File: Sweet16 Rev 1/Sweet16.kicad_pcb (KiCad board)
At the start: 2 copper layers, 140 x 60 mm, 113 parts, among them J1 Conn_01x09_Male, J10 SW_half_inverter, J11 R_clock, J12 OUT_clock, J13 SW_dual8_hex, J14 OUT_OUT, J15 R_sync_pitch_1, J16 SW_sync_1, J17 R_sync_pitch_2, J18 SW_sync_2, J2 Conn_01x09_Male, J20 R_sync_pitch_2, J21 SW_dual8_hex_2, J22 OUT_OUT, J23 OUT_CARRY_OUT, J3 Conn_01x09_Male, J4 Conn_01x09_Male, J5 OUT_OUT, J6 SW_run, J7 SW_BIN_DEC, J8 SW_UP_DN, J9 SW_clock_source, U1 40106, U2 4029, U3 4028, U4 4051, U5 4028, U6 4070, U7 4051, U8 LM358

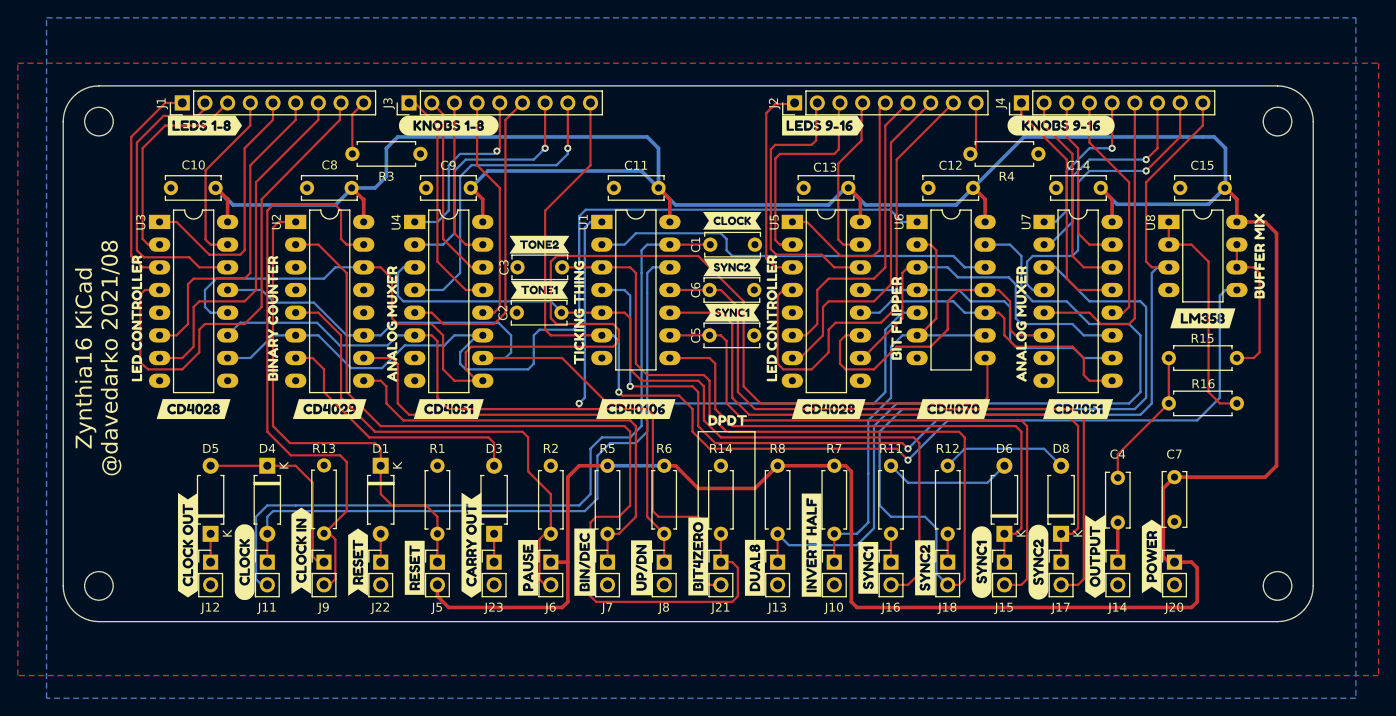
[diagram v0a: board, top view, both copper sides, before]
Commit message: moved the pulldown where it would work
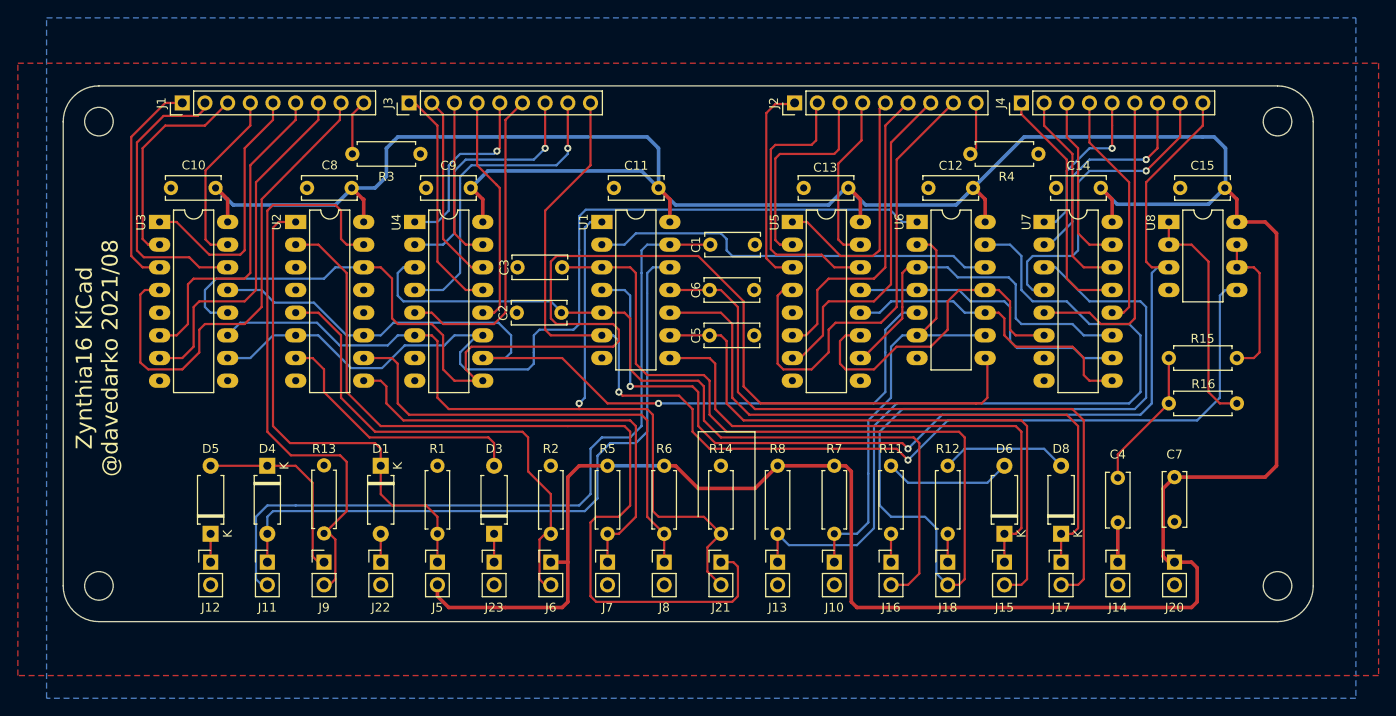
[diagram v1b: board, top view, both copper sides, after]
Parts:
- removed kibuzzard-610C1637, kibuzzard-610C1856, kibuzzard-610C1A63, kibuzzard-610C1AC8, kibuzzard-610C1D73, kibuzzard-610C1E26, kibuzzard-610C2350, kibuzzard-610C23E8, kibuzzard-610C2455, kibuzzard-610C51A7, kibuzzard-610C51E0, kibuzzard-610C523D, kibuzzard-610C5269, kibuzzard-610C52EC, kibuzzard-610C530B, kibuzzard-610C5339, kibuzzard-610C5373, kibuzzard-610C5418, kibuzzard-610C545E, kibuzzard-610C5562, kibuzzard-610C55EA, kibuzzard-610C561B, kibuzzard-6111A8BD, kibuzzard-6112EA2B, kibuzzard-6112EA3D, kibuzzard-6112EA56, kibuzzard-6112EA78, kibuzzard-6112EA8E, kibuzzard-6112EAB9, kibuzzard-6112EAC9, kibuzzard-6112EADF, kibuzzard-6112EDB2, kibuzzard-6112EDD8, kibuzzard-6112EDF7, kibuzzard-6112EE23, kibuzzard-6112EE9D, kibuzzard-6112EEB7, kibuzzard-6112EED9, kibuzzard-6112EEFB, kibuzzard-6112F4A3, kibuzzard-6112F4D1, kibuzzard-6112F4F2, kibuzzard-6112F51D, kibuzzard-6112F530: G***, label
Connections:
- R14 pad 1: QD0 -> QD1
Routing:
- net QD0: track 101.3 -> 98.2 mm
- net QD1: track 105.4 -> 106.3 mm

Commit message: Revert "moved the pulldown where it would work"
This reverts commit ad45cd7af2cd5e29d93eb6355ad2eb9f66b6a434.
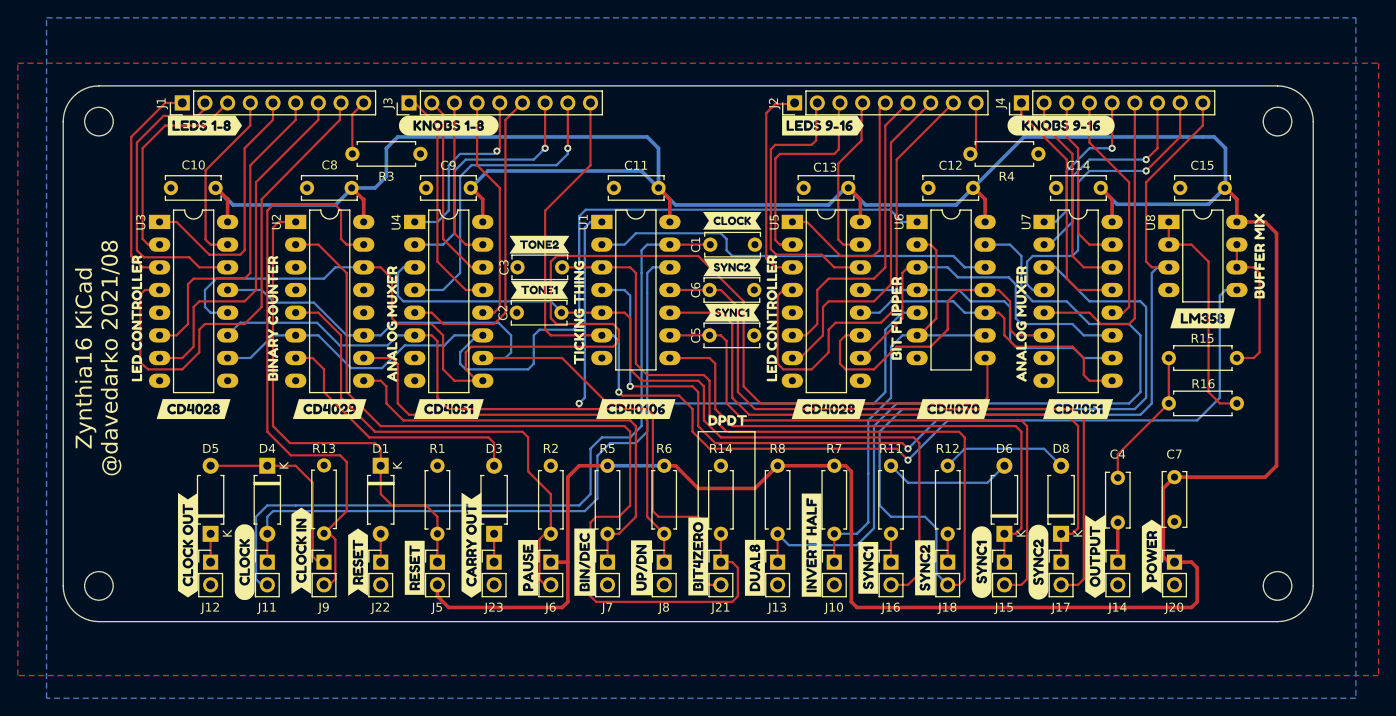
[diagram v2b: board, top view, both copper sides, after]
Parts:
- added kibuzzard-610C1637: G***, label, F.Cu at (45.7, 51.4)
- added kibuzzard-610C1856: G***, label, F.Cu at (64.8, 54.0)
- added kibuzzard-610C1A63: G***, label, F.Cu at (58.4, 53.3)
- added kibuzzard-610C1AC8: G***, label, F.Cu at (83.8, 51.4)
- added kibuzzard-610C1D73: G***, label, F.Cu at (39.4, 54.0)
- added kibuzzard-610C1E26: G***, label, F.Cu at (33.0, 53.3)
- added kibuzzard-610C2350: G***, label, F.Cu at (77.5, 54.0)
- added kibuzzard-610C23E8: G***, label, F.Cu at (71.1, 52.7)
- added kibuzzard-610C2455: G***, label, F.Cu at (74.4, 37.5)
- added kibuzzard-610C51A7: G***, label, F.Cu at (90.2, 54.0)
- added kibuzzard-610C51E0: G***, label, F.Cu at (96.5, 54.0)
- added kibuzzard-610C523D: G***, label, F.Cu at (109.2, 53.3)
- added kibuzzard-610C5269: G***, label, F.Cu at (102.9, 53.3)
- added kibuzzard-610C52EC: G***, label, F.Cu at (15.9, 4.45)
- added kibuzzard-610C530B: G***, label, F.Cu at (85.1, 4.45)
- added kibuzzard-610C5339: G***, label, F.Cu at (111.8, 4.45)
- added kibuzzard-610C5373: G***, label, F.Cu at (43.2, 4.45)
- added kibuzzard-610C5418: G***, label, F.Cu at (14.0, 51.4)
- added kibuzzard-610C545E: G***, label, F.Cu at (26.7, 52.1)
- added kibuzzard-610C5562: G***, label, F.Cu at (20.3, 53.3)
- added kibuzzard-610C55EA: G***, label, F.Cu at (52.1, 54.0)
- added kibuzzard-610C561B: G***, label, F.Cu at (115.6, 52.7)
- added kibuzzard-6111A8BD: G***, label, F.Cu at (121.9, 52.7)
- added kibuzzard-6112EA2B: G***, label, F.Cu at (14.6, 36.2)
- added kibuzzard-6112EA3D: G***, label, F.Cu at (85.7, 36.2)
- added kibuzzard-6112EA56: G***, label, F.Cu at (29.8, 36.2)
- added kibuzzard-6112EA78: G***, label, F.Cu at (43.2, 36.2)
- added kibuzzard-6112EA8E: G***, label, F.Cu at (113.7, 36.2)
- added kibuzzard-6112EAB9: G***, label, F.Cu at (64.1, 36.2)
- added kibuzzard-6112EAC9: G***, label, F.Cu at (99.7, 36.2)
- added kibuzzard-6112EADF: G***, label, F.Cu at (127.6, 26.0)
- added kibuzzard-6112EDB2: G***, label, F.Cu at (8.26, 26.0)
- added kibuzzard-6112EDD8: G***, label, F.Cu at (23.5, 26.0)
- added kibuzzard-6112EDF7: G***, label, F.Cu at (36.8, 26.7)
- added kibuzzard-6112EE23: G***, label, F.Cu at (107.3, 26.7)
- added kibuzzard-6112EE9D: G***, label, F.Cu at (57.8, 25.4)
- added kibuzzard-6112EEB7: G***, label, F.Cu at (79.4, 26.0)
- added kibuzzard-6112EED9: G***, label, F.Cu at (134.0, 19.1)
- added kibuzzard-6112EEFB: G***, label, F.Cu at (93.3, 26.0)
- added kibuzzard-6112F4A3: G***, label, F.Cu at (74.9, 15.1)
- added kibuzzard-6112F4D1: G***, label, F.Cu at (53.3, 22.9)
- added kibuzzard-6112F4F2: G***, label, F.Cu at (53.3, 17.8)
- added kibuzzard-6112F51D: G***, label, F.Cu at (74.9, 25.4)
- added kibuzzard-6112F530: G***, label, F.Cu at (74.9, 20.3)
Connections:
- R14 pad 1: QD1 -> QD0
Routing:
- net QD0: track 98.2 -> 101.3 mm
- net QD1: track 106.3 -> 105.4 mm
